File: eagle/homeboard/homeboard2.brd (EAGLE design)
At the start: 100 x 80 mm, 81 parts, among them IC1 XCF02S, IC2 25LC080SN, Q5 BC848SMD, Q6 BC848SMD, Q7 BC848SMD, Q8 BC848SMD, T1 BSS138, T2 BC848, T3 BSS138, U1 XC3S400TQ144, X1 1503_04, X2 SCART-F

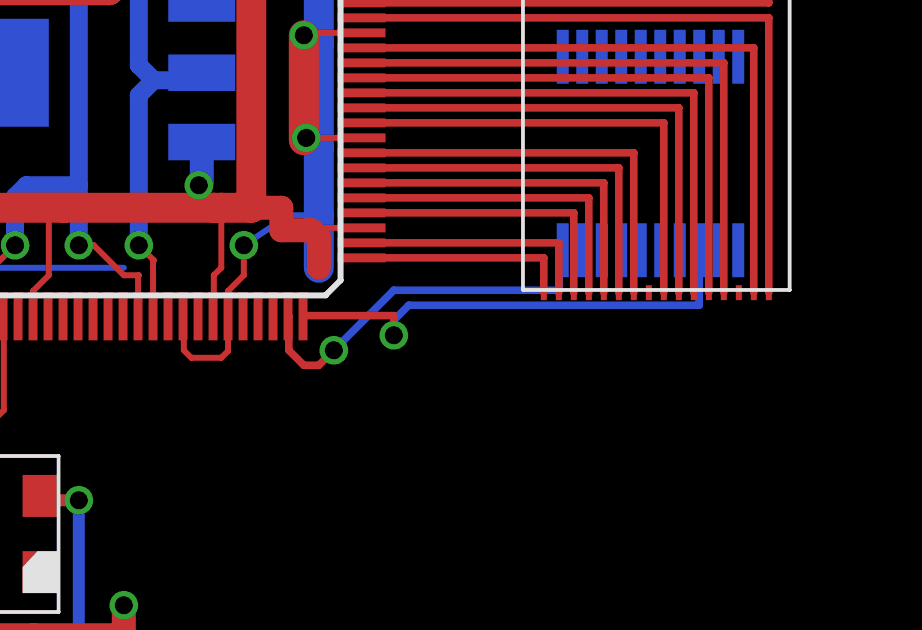
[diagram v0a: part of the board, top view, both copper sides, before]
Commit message: mah
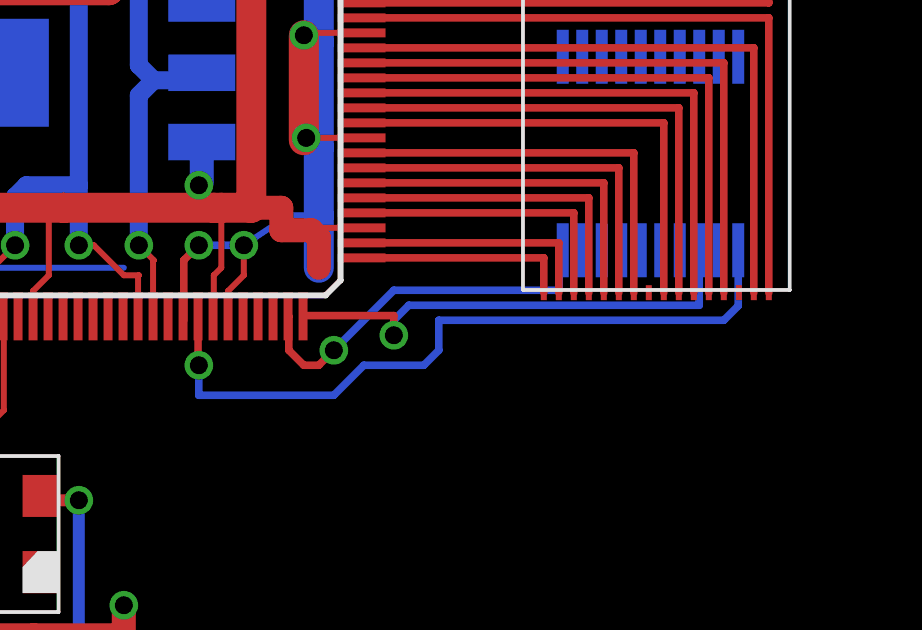
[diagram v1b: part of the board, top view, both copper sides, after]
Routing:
- net PROM_DO: track 0.00 -> 24.3 mm, vias 0 -> 1
- net GND: track 368.1 -> 368.5 mm, vias 19 -> 20
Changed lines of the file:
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@@
 <contactref element="REG2.5" pad="1"/>
 <wire x1="31.525" y1="29.08" x2="24.5" y2="29.08" width="0.2" layer="1"/>
-<wire x1="24.5" y1="29.08" x2="62.5" y2="14.42" width="0" layer="19" extent="1-16"/>
-<wire x1="65.5" y1="14.42" x2="21.5" y2="35" width="0" layer="19" extent="1-16"/>
 <wire x1="21.5" y1="35" x2="22" y2="35.5" width="0.2" layer="1"/>
 <wire x1="24" y1="35.5" x2="24.5" y2="35" width="0.2" layer="1"/>
-<wire x1="24.5" y1="35" x2="62.5" y2="14.42" width="0" layer="19" extent="1-16"/>
 <contactref element="X4" pad="8"/>
 <contactref element="X4" pad="G1"/>
@@
 <wire x1="43.5" y1="1.75" x2="37" y2="1.75" width="1" layer="16"/>
 <wire x1="37" y1="1.75" x2="32" y2="1.75" width="1" layer="16"/>
-<wire x1="48.475" y1="13.63" x2="48.475" y2="12.475" width="0.2" layer="1"/>
-<wire x1="48.475" y1="12.475" x2="48.25" y2="12.25" width="0.2" layer="1"/>
-<wire x1="48.25" y1="12.25" x2="47.25" y2="12.25" width="0.2" layer="1"/>
-<wire x1="47.25" y1="12.25" x2="47" y2="12.5" width="0.2" layer="1"/>
-<wire x1="47" y1="12.5" x2="47" y2="13.5" width="0.2" layer="1"/>
 <wire x1="33.5" y1="25.75" x2="33.5" y2="29.5" width="1" layer="16"/>
-<wire x1="52" y1="4.7164" x2="59.6304" y2="22.2836" width="0" layer="19" extent="1-16"/>
 <wire x1="52" y1="1.75" x2="51.8696" y2="1.75" width="0.4" layer="16"/>
 <wire x1="28.75" y1="7.75" x2="34.5" y2="7.75" width="0.2" layer="16"/>
@@
 <wire x1="42.225" y1="7.645" x2="42.355" y2="7.645" width="0.4" layer="1"/>
 <wire x1="42.355" y1="7.645" x2="42.5" y2="7.5" width="0.4" layer="1"/>
-<wire x1="59.6304" y1="22.2836" x2="51.8696" y2="2.1196" width="0" layer="19" extent="1-16"/>
 <wire x1="51.8696" y1="2.1196" x2="51.5" y2="1.75" width="0.4" layer="16"/>
 <wire x1="36.901" y1="24.689" x2="34.189" y2="24.689" width="1" layer="16"/>
@@
 <wire x1="50.5" y1="17" x2="51.5" y2="17" width="0.2" layer="16"/>
 <wire x1="53.5" y1="35.5" x2="51.5" y2="33.75" width="1" layer="16"/>
-<wire x1="53.5" y1="14.5" x2="52.25" y2="14.5" width="0" layer="19" extent="1-16"/>
-<wire x1="52.25" y1="14.5" x2="51.5" y2="15.25" width="0" layer="19" extent="1-16"/>
 <wire x1="51.5" y1="15.25" x2="51.5" y2="17" width="1" layer="16"/>
 <wire x1="53.5" y1="35.5" x2="52.75" y2="36.25" width="1" layer="16"/>
@@
 <wire x1="32.5" y1="35.5" x2="32.5" y2="34" width="1" layer="16"/>
 <wire x1="32.5" y1="34" x2="33.25" y2="33.25" width="1" layer="16"/>
+<wire x1="47" y1="13.5" x2="47" y2="15.5" width="0.254" layer="1"/>
+<wire x1="47" y1="15.5" x2="47.5" y2="16" width="0.254" layer="1"/>
+<via x="47.5" y="16" extent="1-16" drill="0.6" shape="square"/>
+<wire x1="47.5" y1="16" x2="49" y2="16" width="0.254" layer="16"/>
 <wire x1="96.05" y1="71" x2="95.55" y2="76" width="0" layer="19" extent="1-1"/>
 <wire x1="96.55" y1="67.5" x2="96.05" y2="71" width="0" layer="19" extent="1-1"/>
@@
 <wire x1="11.4778" y1="77" x2="25.3716" y2="78.27" width="0" layer="19" extent="1-1"/>
 <wire x1="1.2" y1="77.75" x2="11.4778" y2="77" width="0" layer="19" extent="1-1"/>
-<wire x1="56.9" y1="44.905" x2="42.4778" y2="77" width="0" layer="19" extent="16-16"/>
-<wire x1="37.475" y1="35.03" x2="56.9" y2="44.905" width="0" layer="19" extent="1-16"/>
+<wire x1="18.25" y1="44.5" x2="11.4778" y2="77" width="0" layer="19" extent="1-1"/>
+<wire x1="7.665" y1="37" x2="7.5" y2="37" width="0" layer="19" extent="1-1"/>
+<wire x1="7.5" y1="10.165" x2="7.5" y2="10" width="0" layer="19" extent="1-1"/>
+<wire x1="34.5" y1="2" x2="35" y2="1.75" width="0" layer="19" extent="16-16"/>
 <wire x1="46.975" y1="13.63" x2="47" y2="13.5" width="0" layer="19" extent="1-1"/>
-<wire x1="7.5" y1="37" x2="7.5" y2="36.835" width="0" layer="19" extent="1-1"/>
-<wire x1="7.5" y1="10.165" x2="7.5" y2="10" width="0" layer="19" extent="1-1"/>
 <wire x1="4.93" y1="35" x2="5" y2="37" width="0" layer="19" extent="1-1"/>
+<wire x1="59.6304" y1="22.2836" x2="52.925" y2="23.08" width="0" layer="19" extent="1-16"/>
+<wire x1="62.5" y1="14.42" x2="59.6304" y2="22.2836" width="0" layer="19" extent="1-16"/>
+<wire x1="65.5" y1="14.42" x2="62.5" y2="14.42" width="0" layer="19" extent="1-1"/>
+<wire x1="56.9" y1="44.905" x2="52.75" y2="36.25" width="0" layer="19" extent="16-16"/>
 </signal>
 <signal name="VCC">
@@
 <contactref element="IC1" pad="1"/>
 <contactref element="U1" pad="P65"/>
-<wire x1="47.475" y1="13.63" x2="65.4804" y2="15.8336" width="0" layer="19" extent="1-16"/>
+<wire x1="65.4804" y1="15.8336" x2="65.4804" y2="13.9804" width="0.254" layer="16"/>
+<wire x1="65.4804" y1="13.9804" x2="65" y2="13.5" width="0.254" layer="16"/>
+<wire x1="65" y1="13.5" x2="55.5" y2="13.5" width="0.254" layer="16"/>
+<wire x1="55.5" y1="13.5" x2="55.5" y2="12.5" width="0.254" layer="16"/>
+<wire x1="55.5" y1="12.5" x2="55" y2="12" width="0.254" layer="16"/>
+<wire x1="55" y1="12" x2="53" y2="12" width="0.254" layer="16"/>
+<wire x1="53" y1="12" x2="52" y2="11" width="0.254" layer="16"/>
+<wire x1="52" y1="11" x2="47.5" y2="11" width="0.254" layer="16"/>
+<wire x1="47.475" y1="13.63" x2="47.475" y2="12.025" width="0.254" layer="1"/>
+<wire x1="47.475" y1="12.025" x2="47.5" y2="12" width="0.254" layer="1"/>
+<via x="47.5" y="12" extent="1-16" drill="0.6" shape="square"/>
+<wire x1="47.5" y1="12" x2="47.5" y2="11" width="0.254" layer="16"/>
 </signal>
 <signal name="VCCINT">
